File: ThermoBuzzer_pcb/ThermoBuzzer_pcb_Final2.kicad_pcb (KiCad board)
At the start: 2 copper layers, 60 x 60 mm, 13 parts, among them SW2 SW_Push

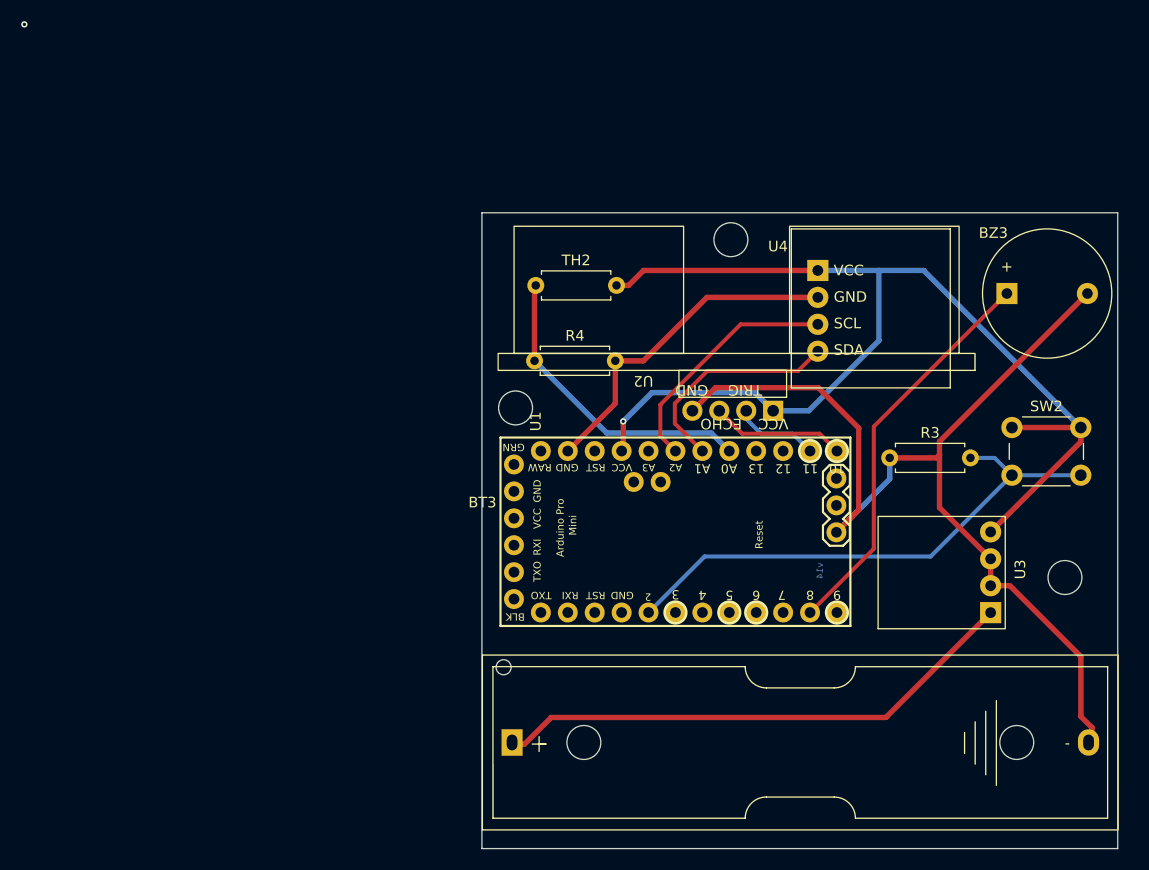
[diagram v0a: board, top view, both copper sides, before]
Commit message: 4.27
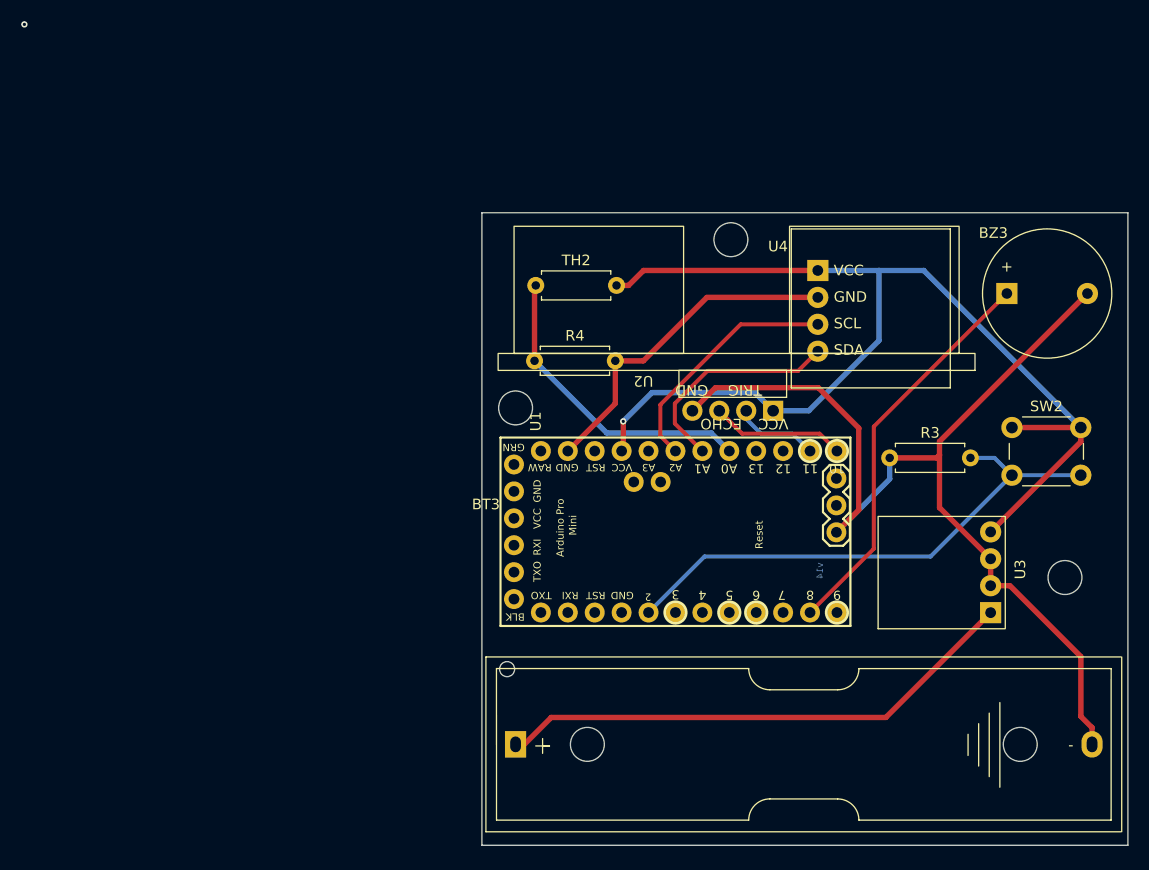
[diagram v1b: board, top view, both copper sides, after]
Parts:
- moved BT3 0.38 mm to (94.4, 110.5)
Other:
- board size 60 x 60 mm -> 61 x 59.7 mm
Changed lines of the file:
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@@
 	(footprint "custom_footprints:6s-aa 14500"
 		(layer "F.Cu")
-		(at 94.0248 110.3172)
+		(at 94.355 110.495)
 		(property "Reference" "BT3"
 			(at 0 -14.4 0)
@@
 	(gr_rect
 		(start 93.98 68.58)
-		(end 153.98 128.58)
+		(end 154.94 128.27)
 		(stroke
 			(width 0.05)
